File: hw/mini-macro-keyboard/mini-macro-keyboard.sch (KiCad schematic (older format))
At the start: 9 parts

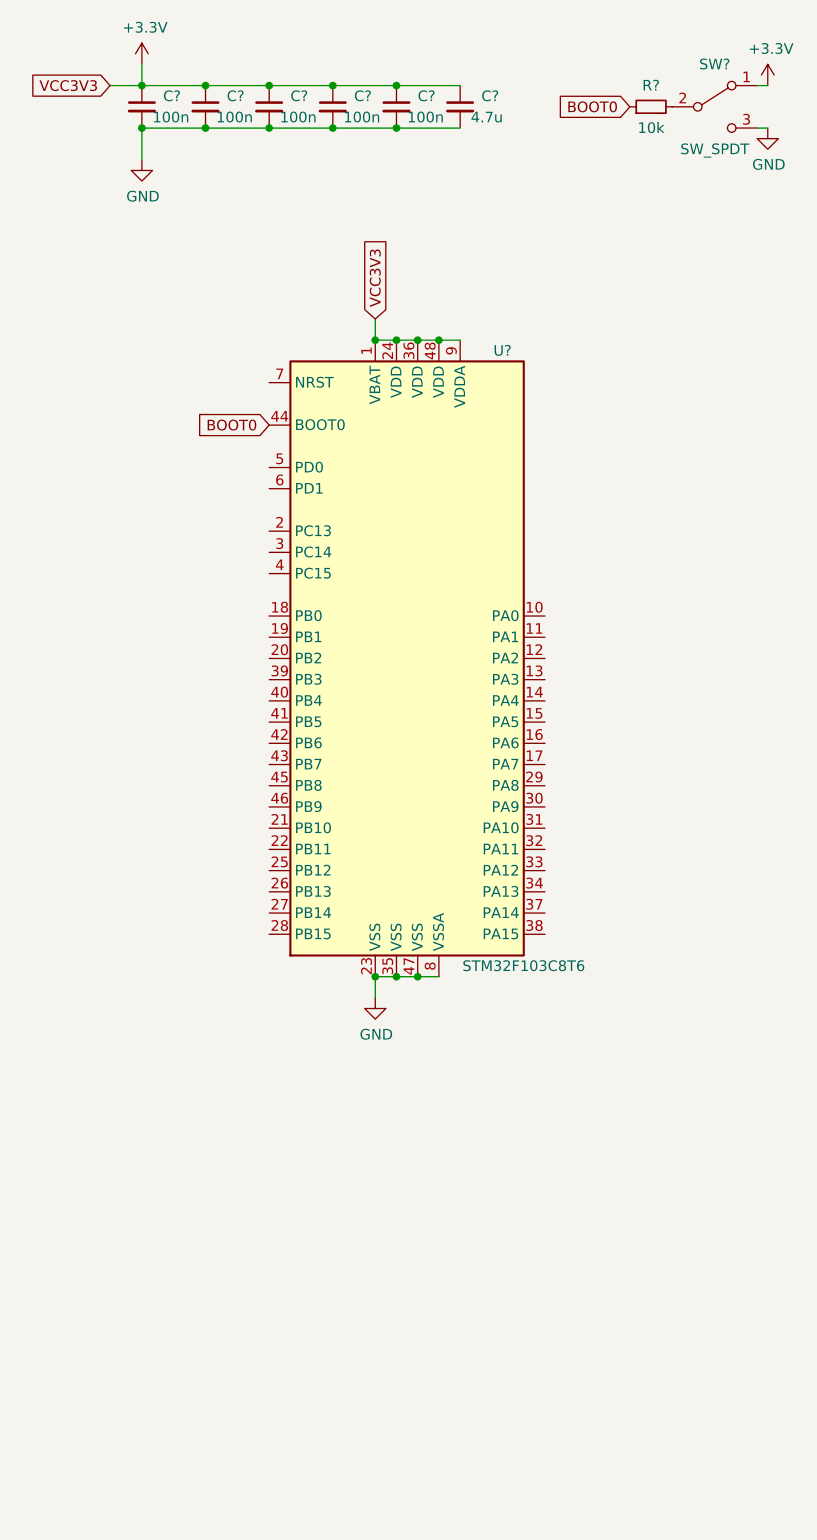
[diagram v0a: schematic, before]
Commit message: feat(hw): add nrst switch
Signed-off-by: Ivan Kovalenko <s1ckretbox@gmail.com>
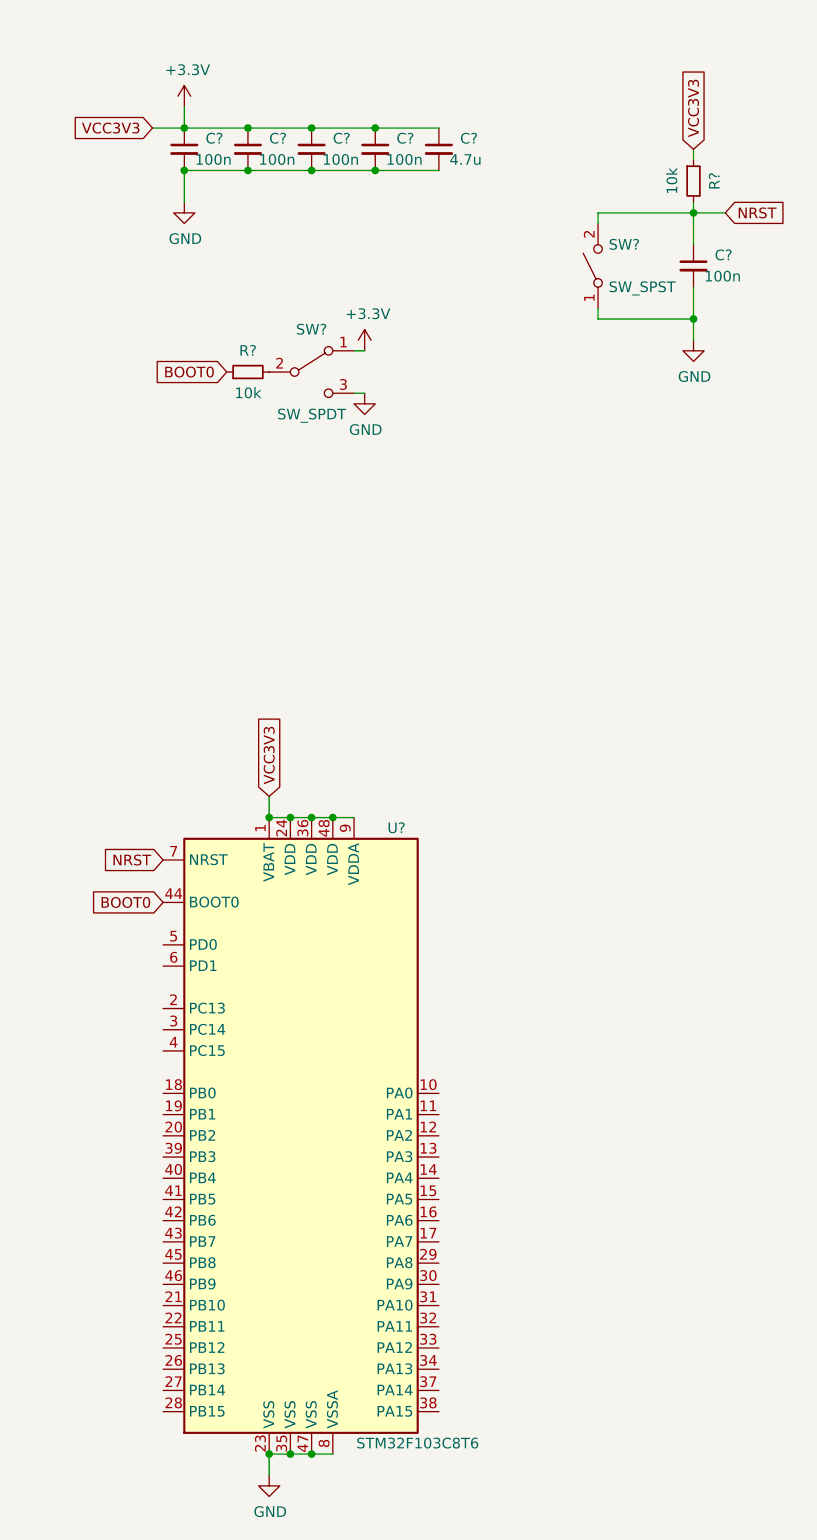
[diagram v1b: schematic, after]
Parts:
- added R?: 10k, symbol Device:R_Small
- added SW?: SW_SPST, symbol Switch:SW_SPST
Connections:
- net +3V3: now also R?.1; no longer C?.1
- net GND: now also SW?.1 (A)
- net NRST: now reaches U?.7 (NRST)
- net NRST: now also C?.1, R?.2, SW?.2 (B)
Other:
- moved on the sheet: C?, R?, SW?, U?
